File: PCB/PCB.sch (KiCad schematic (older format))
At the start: 12 parts, among them J1 USB_B, U1 ESP32-WROOM-32, X1 12MHz

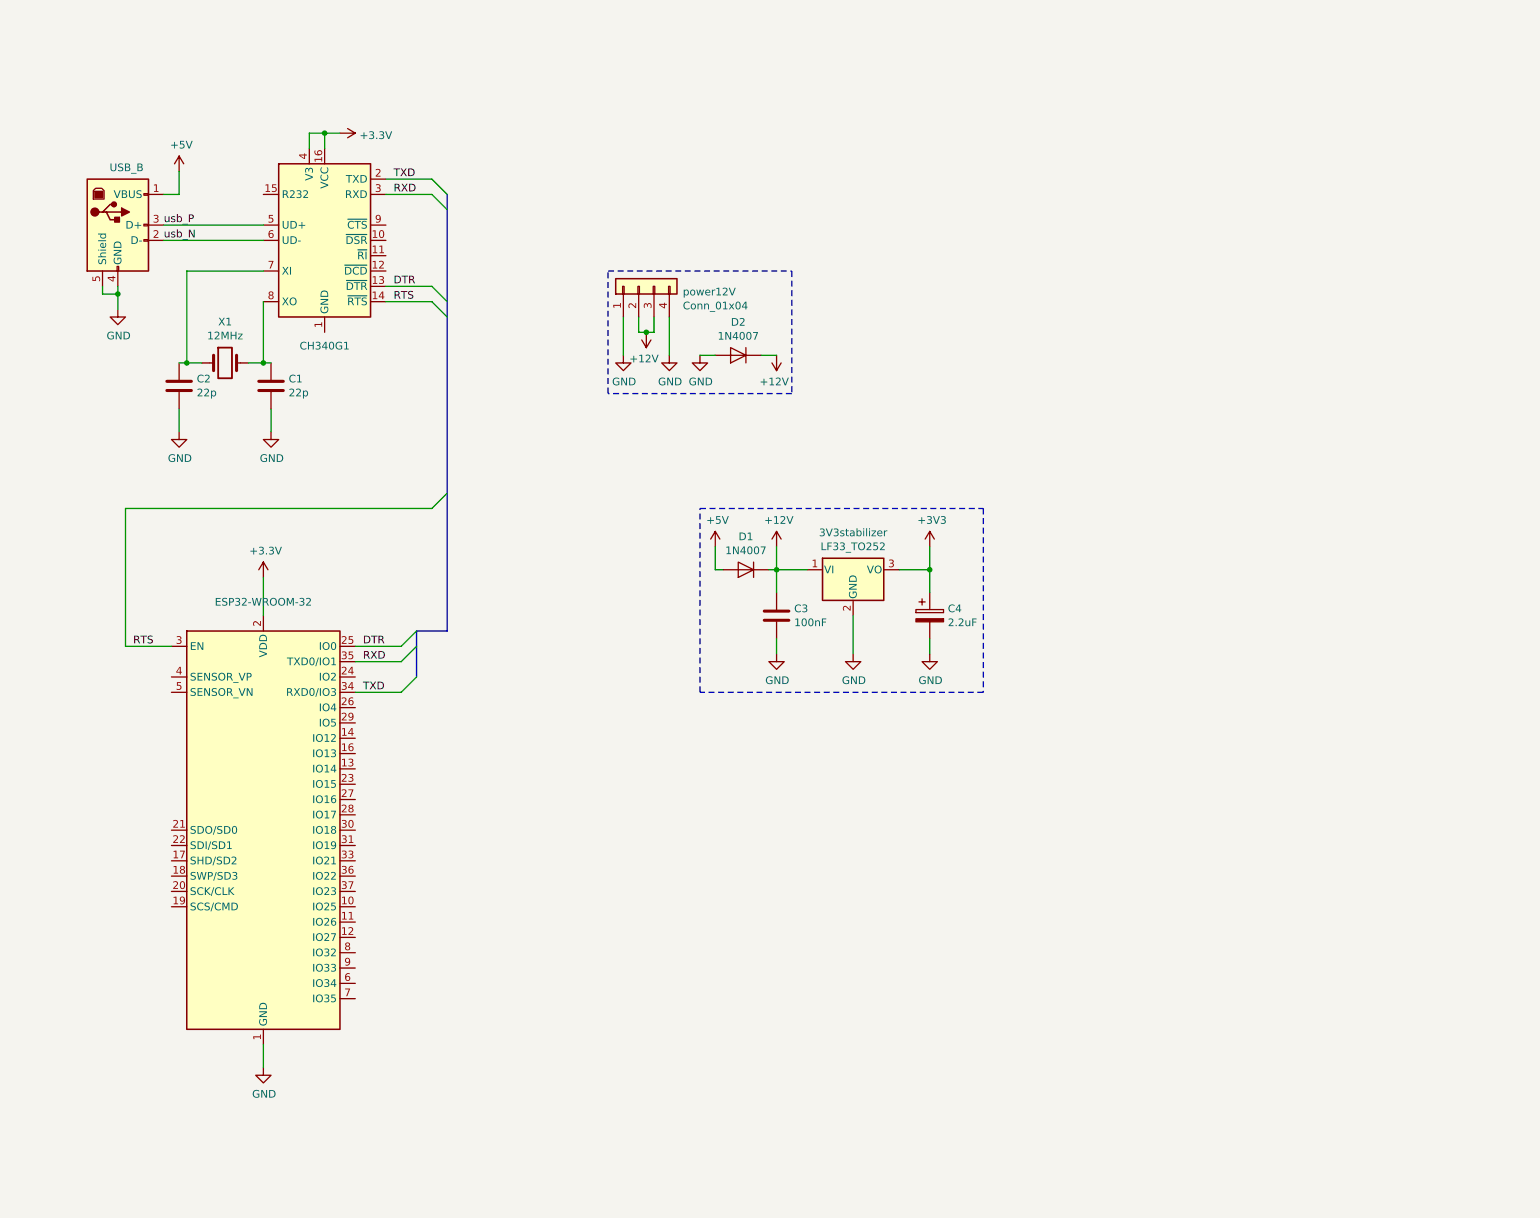
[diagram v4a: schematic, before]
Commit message: pwm fan #4
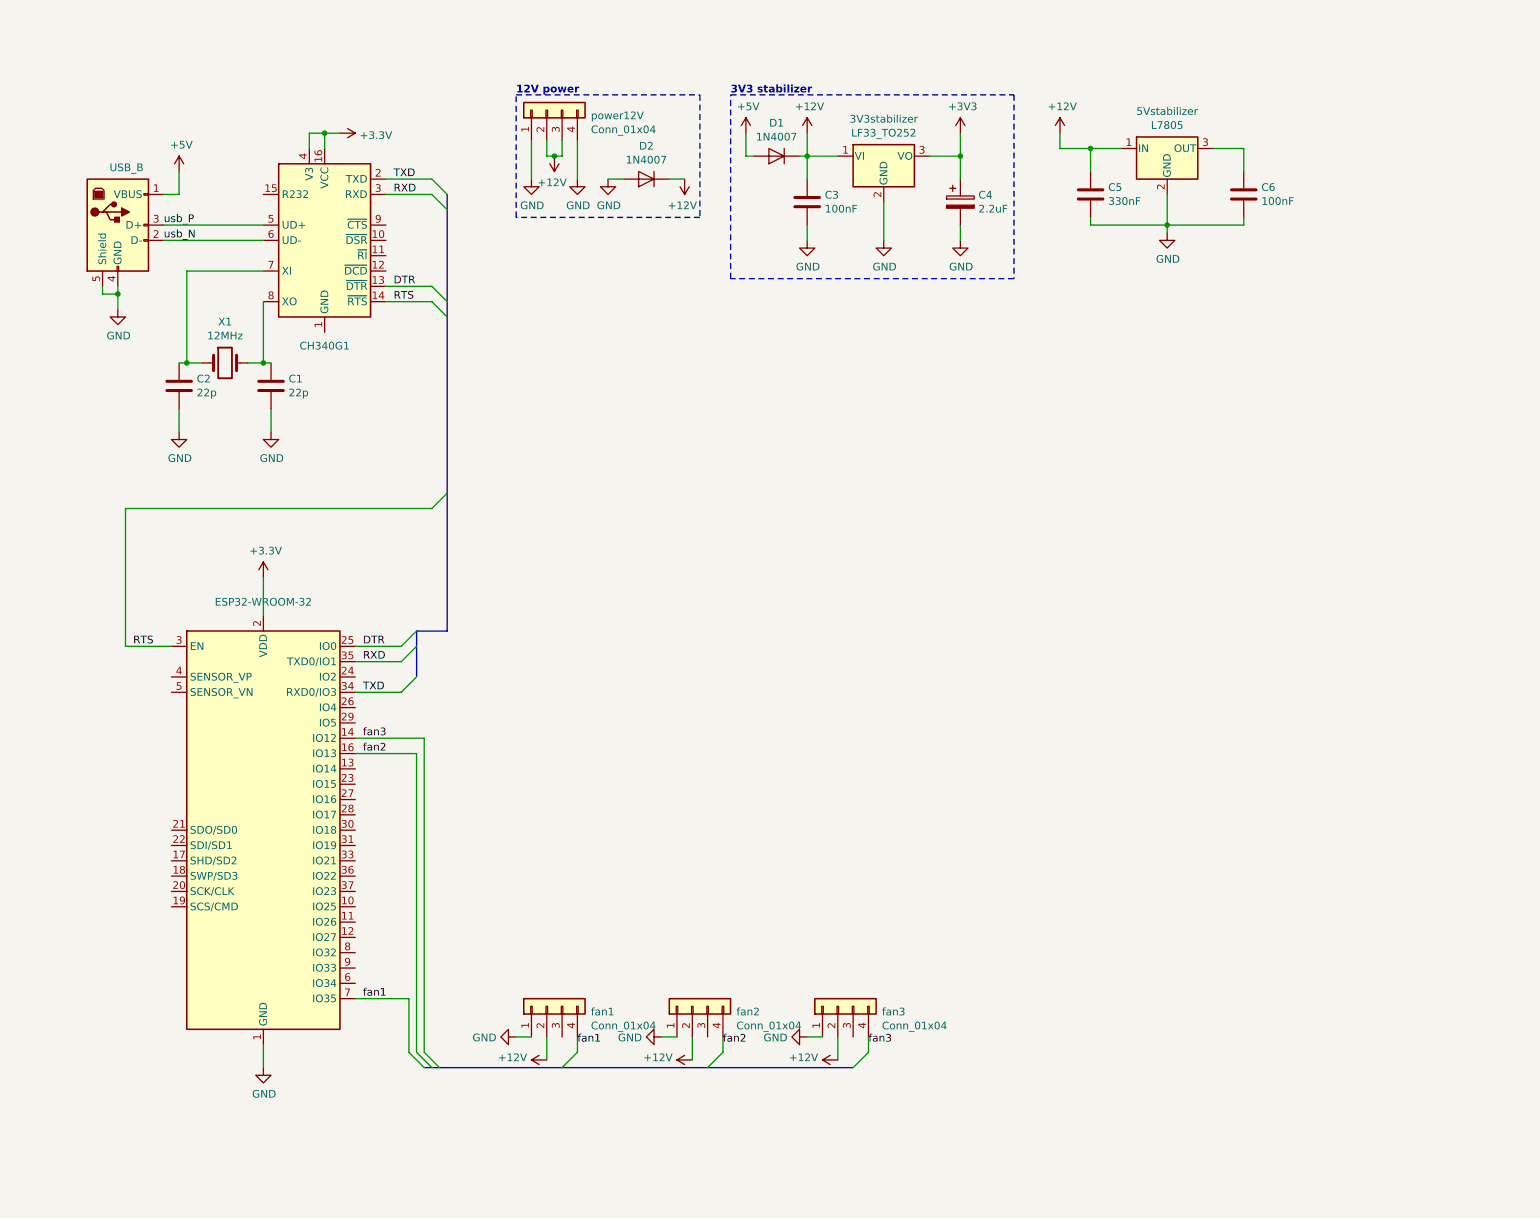
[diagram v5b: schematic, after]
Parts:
- added 5Vstabilizer: L7805, Package_TO_SOT_SMD:TO-252-2, symbol Regulator_Linear:L7805
- added C5: 330nF, symbol Device:C
- added C6: 100nF, symbol Device:C
- added fan1, fan2, fan3: Conn_01x04, Connector:FanPinHeader_1x04_P2.54mm_Vertical, symbol Connector_Generic:Conn_01x04
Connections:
- net +12V: now also 5Vstabilizer.1 (IN), C5.1, fan1.2 (Pin_2), fan2.2 (Pin_2), fan3.2 (Pin_2)
- net GND: now also 5Vstabilizer.2 (GND), C5.2, C6.2, fan1.1 (Pin_1), fan2.1 (Pin_1), fan3.1 (Pin_1)
- net fan3: now reaches U1.14 (IO12)
- net fan3: now also fan3.4 (Pin_4)
- net fan2: now reaches U1.16 (IO13)
- net fan2: now also fan2.4 (Pin_4)
- net fan1: now reaches U1.7 (IO35)
- net fan1: now also fan1.4 (Pin_4)
- new net: 5Vstabilizer.3 (OUT), C6.1
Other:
- note added: "12V power"
- note added: "3V3 stabilizer"
- moved on the sheet: 3V3stabilizer, C3, C4, D1, D2, power12V
